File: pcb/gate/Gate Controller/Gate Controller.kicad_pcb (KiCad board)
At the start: 2 copper layers, 111.2 x 92.8 mm, 53 parts, among them IC1 MCP23009-E_SS, J11 Left Post, J13 AUX, J14 AUX, J17 AUX, J18 Power, J19 Fiber Power, J20 Driveway lights, J21 POE Camera, J23 Right Post, J25 Motor Controller, J26 Ethernet, J28 Pi, J3 CN7, J30 Post, J4 CN1, J6 Safety Stop, J8 Detect Gate Open, J9 Raspberry Controller, K1 EC2-5SNU, P1 pi, Q1 FDC6561AN, Q2 FDC6561AN, Q3 FDC6561AN, T1 STD40NF10

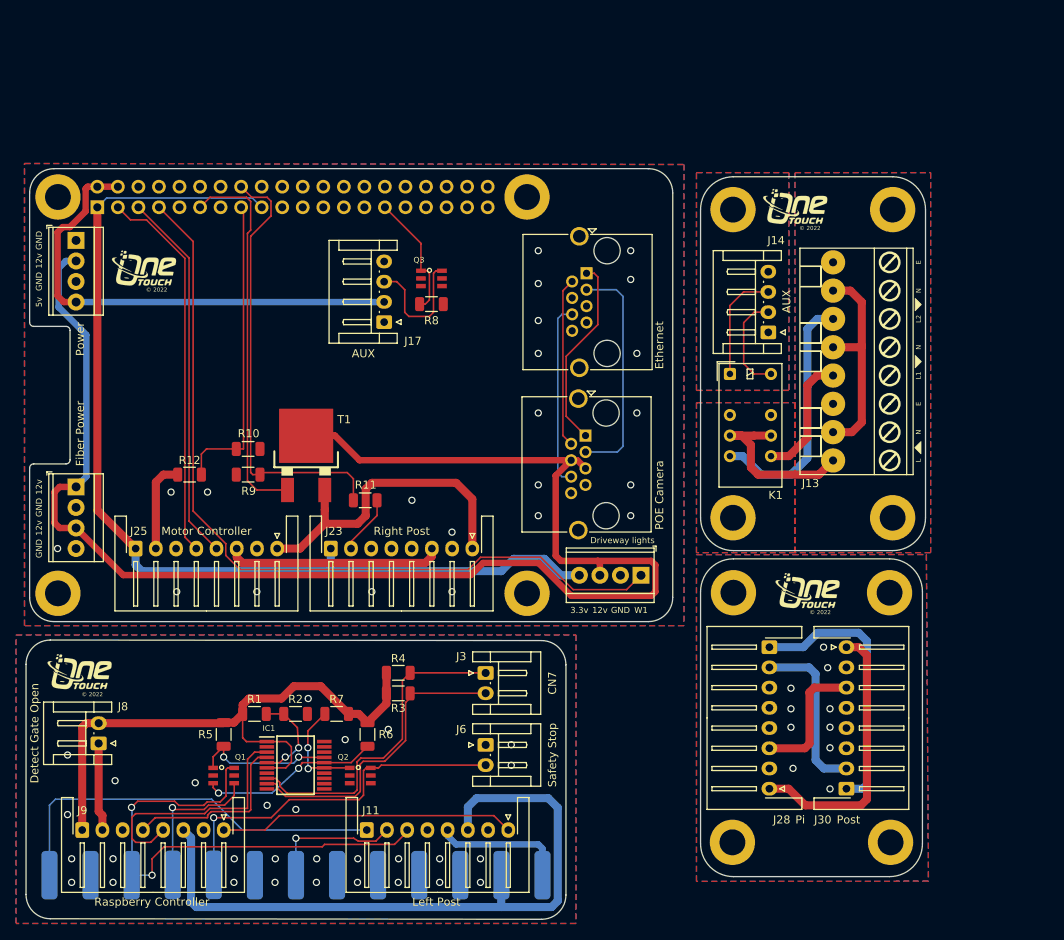
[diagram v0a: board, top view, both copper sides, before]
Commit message: latest updates
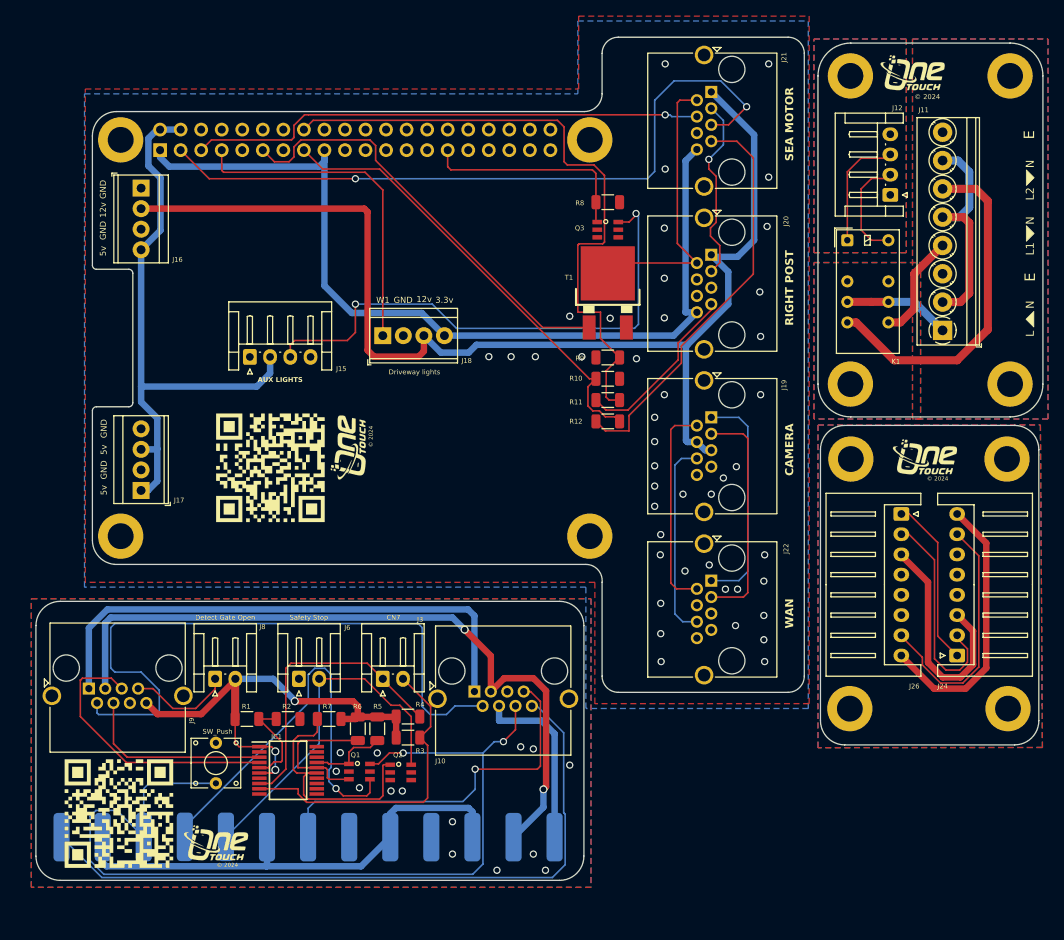
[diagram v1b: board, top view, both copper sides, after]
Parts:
- removed J13: AUX, TerminalBlock_Phoenix:TerminalBlock_Phoenix_PT_1.5-8-PVH-3.5
- removed J14: AUX, Connector_JST:JST_EH_S4B-EH_1x04_P2.50mm_Horizontal
- removed J23: Right Post, Connector_JST:JST_XH_PinSWAP
- removed J25: Motor Controller, Connector_JST:JST_XH_PinSWAP
- removed J28: Pi, Connector_JST:JST_XH_PinSWAP
- removed J30: Post, Connector_JST:JST_XH_PinSWAP
- added J10: RJ45_Shielded, Connector_RJ:RJ45_Amphenol_RJHSE5380, F.Cu at (108.2, 175.9)
- added J12: AUX, Connector_JST:JST_EH_S4B-EH_1x04_P2.50mm_Horizontal, F.Cu at (159.6, 114.5)
- added J15: AUX, Connector_JST:JST_EH_S4B-EH_1x04_P2.50mm_Horizontal, F.Cu at (80.5, 134.5)
- added J16: Power, TerminalBlock_TE-Connectivity:TerminalBlock_TE_282834-4_1x04_P2.54mm_Horizontal, F.Cu at (67.0, 113.7)
- added J22: Ethernet, Connector_RJ:RJ45_Amphenol_RJHSE5380, F.Cu at (137.5, 162.2)
- added J24: Pi, Connector_JST:JST_XH_S8B-XH-A_1x08_P2.50mm_Horizontal, F.Cu at (167.9, 171.4)
- added SW4: SW_Push, Button_Switch_THT:TS-D015, F.Cu at (76.2, 184.8)
- added U1: ~, Logos:QRCode Github Automation, F.Cu at (57.3, 198.0)
- added U2: ~, Logos:QRCode Github Automation, F.Cu at (90.0, 155.2)
- J11: value Left Post -> AUX; footprint Connector_JST:JST_XH_PinSWAP -> TerminalBlock_Phoenix:TerminalBlock_Phoenix_PT-1,5-8-3.5-H_1x08_P3.50mm_Horizontal
- J17: value AUX -> Fiber Power; footprint Connector_JST:JST_EH_S4B-EH_1x04_P2.50mm_Horizontal -> TerminalBlock_TE-Connectivity:TerminalBlock_TE_282834-4_1x04_P2.54mm_Horizontal
- J18: value Power -> Driveway lights
- J19: value Fiber Power -> POE Camera; footprint TerminalBlock_TE-Connectivity:TerminalBlock_TE_282834-4_1x04_P2.54mm_Horizontal -> Connector_RJ:RJ45_Amphenol_RJHSE5380
- J20: value Driveway lights -> RJ45_Shielded; footprint TerminalBlock_TE-Connectivity:TerminalBlock_TE_282834-4_1x04_P2.54mm_Horizontal -> Connector_RJ:RJ45_Amphenol_RJHSE5380
- J21: value POE Camera -> RJ45_Shielded
- J26: value Ethernet -> Post; footprint Connector_RJ:RJ45_Amphenol_RJHSE5380 -> Connector_JST:JST_XH_S8B-XH-A_1x08_P2.50mm_Horizontal
- J9: value Raspberry Controller -> RJ45_Shielded; footprint Connector_JST:JST_XH_PinSWAP -> Connector_RJ:RJ45_Amphenol_RJHSE5380
- moved J11 81.9 mm to (166.1, 131.2), turned to 90 degrees
- moved J19 79.0 mm to (137.5, 142.0)
- moved R12 52.1 mm to (124.7, 142.5)
- moved J26 49.0 mm to (161.0, 153.9)
- moved R9 46.8 mm to (124.7, 134.6)
- moved R10 45.3 mm to (124.7, 137.2)
- moved J21 45.2 mm to (137.5, 101.8)
- moved T1 42.4 mm to (124.7, 127.6)
- moved J20 40.6 mm to (137.5, 121.9), turned to -90 degrees
- moved J18 39.7 mm to (96.9, 131.9), turned to 0 degrees
- moved J17 36.6 mm to (67.0, 151.0)
- moved G3 33.7 mm to (92.8, 145.8), turned to 90 degrees
- moved R11 32.4 mm to (124.7, 139.9), turned to 180 degrees
- moved G1 27.1 mm to (76.2, 194.8)
- moved R8 25.2 mm to (124.7, 115.4)
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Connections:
- J11 pad 1: GATE_LED_12V -> L
- J11 pad 2: GND -> N
- J11 pad 3: CN1_24v(FL) -> E
- J11 pad 4: CN1_(FL)- -> L1
- J11 pad 5: GND -> N
- J11 pad 6: START -> L2
- J11 pad 7: PH1 -> N
- J11 pad 8: ANTENNA+ -> E
- J17 pad 1: GND -> +5v
- J17 pad 2: 5v -> GND
- J17 pad 3: Net-(J17-Pad3) -> +5v
- J18 pad 1: GND -> W1
- J18 pad 2: +12V -> GND
- J18 pad 3: GND -> +12V
- J18 pad 4: 5v -> 3V3
- J19 pad 1: +12V -> Net-(J19-Pad1)
- J19 pad 2: GND -> Net-(J19-Pad2)
- J19 pad 3: +12V -> Net-(J19-Pad3)
- J19 pad 4: GND -> +12V
- J20 pad 1: W1 -> +12V
- J20 pad 2: GND -> GATE_LED_COM
- J20 pad 3: +12V -> CN1_24v(FL)
- J20 pad 4: 3V3 -> unconnected-(J20-Pad4)
- J21 pad 1: Net-(J21-Pad1) -> +12V
- J21 pad 2: Net-(J21-Pad2) -> GATE_LED_COM
- J21 pad 3: Net-(J21-Pad3) -> CN1_24v(FL)
- J21 pad 4: +12V -> SCL1
- J21 pad 5: +12V -> SDA1
- J21 pad 6: Net-(J21-Pad6) -> GND
- J21 pad 7: GND -> REED LEFT
- J21 pad 8: GND -> 3V3
- J26 pad 1: Net-(J21-Pad1) -> GATE_LED_12V
- J26 pad 2: Net-(J21-Pad2) -> Net-(J24-Pin_2)
- J26 pad 3: Net-(J21-Pad3) -> CN1_24v(FL)
- J26 pad 6: Net-(J21-Pad6) -> GND
- J26 pad 7: unconnected-(J26-Pad7) -> REED RIGHT
- J26 pad 8: unconnected-(J26-Pad8) -> 3V3
- J9 pad 1: GATE_LED_12V -> +12v
- J9 pad 2: GND -> GATE_LED_COM
- P1 pad 2: 5v -> +5v
- P1 pad 4: 5v -> +5v
- Q3 pad 6: Net-(J17-Pad3) -> Net-(J15-Pin_3)
- T1 pad 2: +12V -> GATE_LED_COM
- T1 pad 3: GATE_LED_12V -> GND
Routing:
- net GATE_LED_COM: track 0.00 -> 115.8 mm
- net GATE_LED_12V: track 111.2 -> 20.9 mm, vias 0 -> 1
- net +5v: track 0.00 -> 72.4 mm
- net Net-(J15-Pin_3): track 0.00 -> 66.7 mm, vias 0 -> 2
- net +12v: track 0.00 -> 65.8 mm
- net GND: track 0.00 -> 60.7 mm, vias 61 -> 57
- net W1: track 101.5 -> 41.4 mm
- net 5v: track 60.0 -> 0.00 mm
- net SDA1: track 69.8 -> 123.1 mm, vias 0 -> 2
- net START: track 63.2 -> 115.2 mm
- net REED LEFT: track 22.2 -> 63.6 mm
- net +12V: track 184.6 -> 145.0 mm
- net ANTENNA+: track 49.8 -> 86.7 mm
- net PEDST: track 18.3 -> 50.8 mm
- net 3V3: track 235.0 -> 204.6 mm, vias 0 -> 3
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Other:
- board size 111.2 x 92.8 mm -> 124.5 x 104.2 mm
- board text added: "AUX LIGHTS"
- board text added: "CAMERA"
- board text added: "RIGHT POST"
- board text added: "SEA MOTOR"
- board text added: "WAN"
- board text added: "© 2024"
- board text removed: "© 2022"
